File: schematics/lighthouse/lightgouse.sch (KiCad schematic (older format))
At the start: 4 parts

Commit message: lighthouse scheme
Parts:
- added D1, D2: LED, LEDs:LED-5MM, symbol LED
- added P1: 3V3, Pin_Headers:Pin_Header_Straight_1x01, symbol CONN_01X01
- added P2: GND, Pin_Headers:Pin_Header_Straight_1x01, symbol CONN_01X01
- added R1, R2: 1k, Resistors_ThroughHole:Resistor_Horizontal_RM7mm, symbol R
- added R5: 10k, w_pth_resistors:RC05, symbol R
- R3: renamed from 10k; value R -> 10K; footprint (none) -> w_pth_resistors:RC05
- R4: renamed from 10k; value R -> 10k; footprint (none) -> w_pth_resistors:RC05
- U1: renamed from U?; footprint (none) -> bugs:ESP201
- U2: renamed from U?; footprint (none) -> bugs:RC522
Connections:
- net labels removed: +3V3, GND
- wire segments 31 -> 41
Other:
- moved on the sheet: R3, R4, U2
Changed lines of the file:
@@
 EESchema Schematic File Version 2
+LIBS:lightgouse-rescue
 LIBS:power
 LIBS:device
@@
 $EndDescr
 $Comp
-L rc522 U?
+L rc522 U2
 U 1 1 5718CF80
-P 5250 2900
-F 0 "U?" H 5550 2950 60  0000 C CNN
-F 1 "rc522" H 5550 3100 60  0000 C CNN
-F 2 "" H 5150 3100 60  0000 C CNN
-F 3 "" H 5150 3100 60  0000 C CNN
-	1    5250 2900
+P 5800 2900
+F 0 "U2" H 6100 2950 60  0000 C CNN
+F 1 "rc522" H 6100 3100 60  0000 C CNN
+F 2 "bugs:RC522" H 5700 3100 60  0001 C CNN
+F 3 "" H 5700 3100 60  0000 C CNN
+	1    5800 2900
 	1    0    0    -1
 $EndComp
 $Comp
-L ESP-201 U?
+L R R4
+U 1 1 5718DD6D
+P 4000 3150
+F 0 "R4" V 3900 3150 50  0000 C CNN
+F 1 "10k" V 4000 3150 50  0000 C CNN
+F 2 "w_pth_resistors:RC05" V 3930 3150 50  0001 C CNN
+F 3 "" H 4000 3150 50  0000 C CNN
+	1    4000 3150
+	0    1    1    0
+$EndComp
+$Comp
+L R R3
+U 1 1 5718DDEA
+P 4000 2650
+F 0 "R3" V 4080 2650 50  0000 C CNN
+F 1 "10K" V 4000 2650 50  0000 C CNN
+F 2 "w_pth_resistors:RC05" V 3930 2650 50  0001 C CNN
+F 3 "" H 4000 2650 50  0000 C CNN
+	1    4000 2650
+	0    1    1    0
+$EndComp
+$Comp
+L R R5
+U 1 1 571A5ED5
+P 4000 3250
+F 0 "R5" V 4080 3250 50  0000 C CNN
+F 1 "10k" V 4000 3250 50  0000 C CNN
+F 2 "w_pth_resistors:RC05" V 3930 3250 50  0001 C CNN
+F 3 "" H 4000 3250 50  0000 C CNN
+	1    4000 3250
+	0    1    1    0
+$EndComp
+$Comp
+L CONN_01X01 P1
+U 1 1 571A6BF5
+P 3050 1350
+F 0 "P1" H 3050 1450 50  0000 C CNN
+F 1 "3V3" V 3150 1350 50  0000 C CNN
+F 2 "Pin_Headers:Pin_Header_Straight_1x01" H 3050 1350 50  0001 C CNN
+F 3 "" H 3050 1350 50  0000 C CNN
+	1    3050 1350
+	0    -1   -1   0
+$EndComp
+$Comp
+L CONN_01X01 P2
+U 1 1 571A6C6D
+P 3350 1350
+F 0 "P2" H 3350 1450 50  0000 C CNN
+F 1 "GND" V 3450 1350 50  0000 C CNN
+F 2 "Pin_Headers:Pin_Header_Straight_1x01" H 3350 1350 50  0001 C CNN
+F 3 "" H 3350 1350 50  0000 C CNN
+	1    3350 1350
+	0    -1   -1   0
+$EndComp
+$Comp
+L LED D2
+U 1 1 571A6EF4
+P 2050 3200
+F 0 "D2" H 2050 3300 50  0000 C CNN
+F 1 "LED" H 2050 3100 50  0000 C CNN
+F 2 "LEDs:LED-5MM" H 2050 3200 50  0001 C CNN
+F 3 "" H 2050 3200 50  0000 C CNN
+	1    2050 3200
+	0    1    1    0
+$EndComp
+$Comp
+L LED D1
+U 1 1 571A6FA0
+P 2150 2450
+F 0 "D1" H 2150 2550 50  0000 C CNN
+F 1 "LED" H 2150 2350 50  0000 C CNN
+F 2 "LEDs:LED-5MM" H 2150 2450 50  0001 C CNN
+F 3 "" H 2150 2450 50  0000 C CNN
+	1    2150 2450
+	0    1    1    0
+$EndComp
+$Comp
+L R R2
+U 1 1 571A710A
+P 2400 2650
+F 0 "R2" V 2480 2650 50  0000 C CNN
+F 1 "1k" V 2400 2650 50  0000 C CNN
+F 2 "Resistors_ThroughHole:Resistor_Horizontal_RM7mm" V 2330 2650 50  0001 C CNN
+F 3 "" H 2400 2650 50  0000 C CNN
+	1    2400 2650
+	0    1    1    0
+$EndComp
+$Comp
+L R R1
+U 1 1 571A724A
+P 2350 3450
+F 0 "R1" V 2430 3450 50  0000 C CNN
+F 1 "1k" V 2350 3450 50  0000 C CNN
+F 2 "Resistors_ThroughHole:Resistor_Horizontal_RM7mm" V 2280 3450 50  0001 C CNN
+F 3 "" H 2350 3450 50  0000 C CNN
+	1    2350 3450
+	0    1    1    0
+$EndComp
+$Comp
+L ESP-201 U1
 U 1 1 5718D2DA
 P 3200 3150
-F 0 "U?" H 3300 3300 60  0000 C CNN
+F 0 "U1" H 3300 3300 60  0000 C CNN
 F 1 "ESP-201" H 3200 3450 60  0000 C CNN
-F 2 "" H 3450 3350 60  0000 C CNN
+F 2 "bugs:ESP201" H 3450 3350 60  0001 C CNN
 F 3 "" H 3450 3350 60  0000 C CNN
 	1    3200 3150
@@
 	4700 2550 4700 1950
 Wire Wire Line
-	4700 1950 2200 1950
-Wire Wire Line
-	2200 1950 2200 2750
-Wire Wire Line
-	2200 2750 2600 2750
-Wire Wire Line
-	3800 2750 4700 2750
+	4700 1950 1950 1950
+Wire Wire Line
+	1950 1950 1950 2750
+Wire Wire Line
+	1950 2750 2600 2750
+Wire Wire Line
+	3800 2750 5250 2750
 Wire Wire Line
 	3800 2950 4400 2950
 Wire Wire Line
-	3800 2850 4700 2850
-Wire Wire Line
-	4700 3900 4700 3250
-Wire Wire Line
-	2600 3900 4700 3900
+	3800 2850 5250 2850
+Wire Wire Line
+	4950 3900 4950 3250
+Wire Wire Line
+	2600 3900 4950 3900
 Wire Wire Line
 	2600 3900 2600 3650
 Wire Wire Line
+	4350 3050 4350 3550
+Wire Wire Line
+	4350 3550 3800 3550
+Wire Wire Line
+	3050 1550 3050 2300
+Wire Wire Line
+	3350 1550 3350 2300
+Wire Wire Line
+	4550 3150 5250 3150
+Wire Wire Line
+	4250 2150 4250 3250
+Wire Wire Line
+	5250 2550 4700 2550
+Wire Wire Line
+	4250 3250 4150 3250
+Wire Wire Line
+	4250 3150 4150 3150
+Wire Wire Line
+	3850 3150 3800 3150
+Wire Wire Line
+	3800 3250 3850 3250
+Connection ~ 4250 3150
+Connection ~ 3050 2150
+Wire Wire Line
+	2550 2650 2600 2650
+Wire Wire Line
+	2050 2200 4150 2200
+Wire Wire Line
+	4150 2200 4150 2650
+Connection ~ 3350 2200
+Wire Wire Line
+	3850 2650 3800 2650
+Wire Wire Line
+	3050 2150 4250 2150
+Wire Wire Line
+	2050 3000 2050 2200
+Connection ~ 2150 2200
+Wire Wire Line
+	4550 3450 3800 3450
+Wire Wire Line
+	4550 3150 4550 3450
+Wire Wire Line
+	2500 3450 2600 3450
+Wire Wire Line
+	2550 3550 2600 3550
+Wire Wire Line
+	2050 3450 2200 3450
+Wire Wire Line
+	2050 3400 2050 3450
+Wire Wire Line
+	2150 2250 2150 2200
+Wire Wire Line
+	2250 2650 2150 2650
+Wire Wire Line
 	4400 2950 4400 2650
 Wire Wire Line
-	4400 2650 4700 2650
-Wire Wire Line
-	4700 3050 3950 3050
-Wire Wire Line
-	3950 3050 3950 3550
-Wire Wire Line
-	3950 3550 3800 3550
-$Comp
-L +3V3 #PWR?
-U 1 1 5718DC65
-P 3050 1650
-F 0 "#PWR?" H 3050 1500 50  0001 C CNN
-F 1 "+3V3" H 3050 1790 50  0000 C CNN
-F 2 "" H 3050 1650 50  0000 C CNN
-F 3 "" H 3050 1650 50  0000 C CNN
-	1    3050 1650
-	1    0    0    -1
-$EndComp
-Wire Wire Line
-	3050 1650 3050 2300
-$Comp
-L GND #PWR?
-U 1 1 5718DCCC
-P 3350 1650
-F 0 "#PWR?" H 3350 1400 50  0001 C CNN
-F 1 "GND" H 3350 1500 50  0000 C CNN
-F 2 "" H 3350 1650 50  0000 C CNN
-F 3 "" H 3350 1650 50  0000 C CNN
-	1    3350 1650
-	-1   0    0    1
-$EndComp
-Wire Wire Line
-	3350 1650 3350 2300
-Wire Wire Line
-	4750 3150 4200 3150
-Wire Wire Line
-	4200 3150 4200 3850
-Wire Wire Line
-	4200 3850 2500 3850
-Wire Wire Line
-	2500 3850 2500 3450
-Wire Wire Line
-	2500 3450 2600 3450
-$Comp
-L R 10k
-U 1 1 5718DD6D
-P 2850 1800
-F 0 "10k" V 2930 1800 50  0000 C CNN
-F 1 "R" V 2850 1800 50  0000 C CNN
-F 2 "" V 2780 1800 50  0000 C CNN
-F 3 "" H 2850 1800 50  0000 C CNN
-	1    2850 1800
-	0    1    1    0
-$EndComp
-Wire Wire Line
-	3000 1800 3050 1800
-Connection ~ 3050 1800
-Wire Wire Line
-	3800 3150 3900 3150
-Wire Wire Line
-	3900 3150 3900 1350
-Wire Wire Line
-	3900 1350 2650 1350
-Wire Wire Line
-	2650 1350 2650 1800
-Wire Wire Line
-	2650 1800 2700 1800
-$Comp
-L R 10k
-U 1 1 5718DDEA
-P 3550 1800
-F 0 "10k" V 3630 1800 50  0000 C CNN
-F 1 "R" V 3550 1800 50  0000 C CNN
-F 2 "" V 3480 1800 50  0000 C CNN
-F 3 "" H 3550 1800 50  0000 C CNN
-	1    3550 1800
-	0    1    1    0
-$EndComp
-Wire Wire Line
-	3400 1800 3350 1800
-Connection ~ 3350 1800
-Wire Wire Line
-	3700 1800 3800 1800
-Wire Wire Line
-	3800 1800 3800 2650
+	4400 2650 5250 2650
+Wire Wire Line
+	4350 3050 5250 3050
+Wire Wire Line
+	5250 3250 5150 3250
+Wire Wire Line
+	5150 3250 5150 1750
+Wire Wire Line
+	5150 1750 3050 1750
+Connection ~ 3050 1750
 $EndSCHEMATC

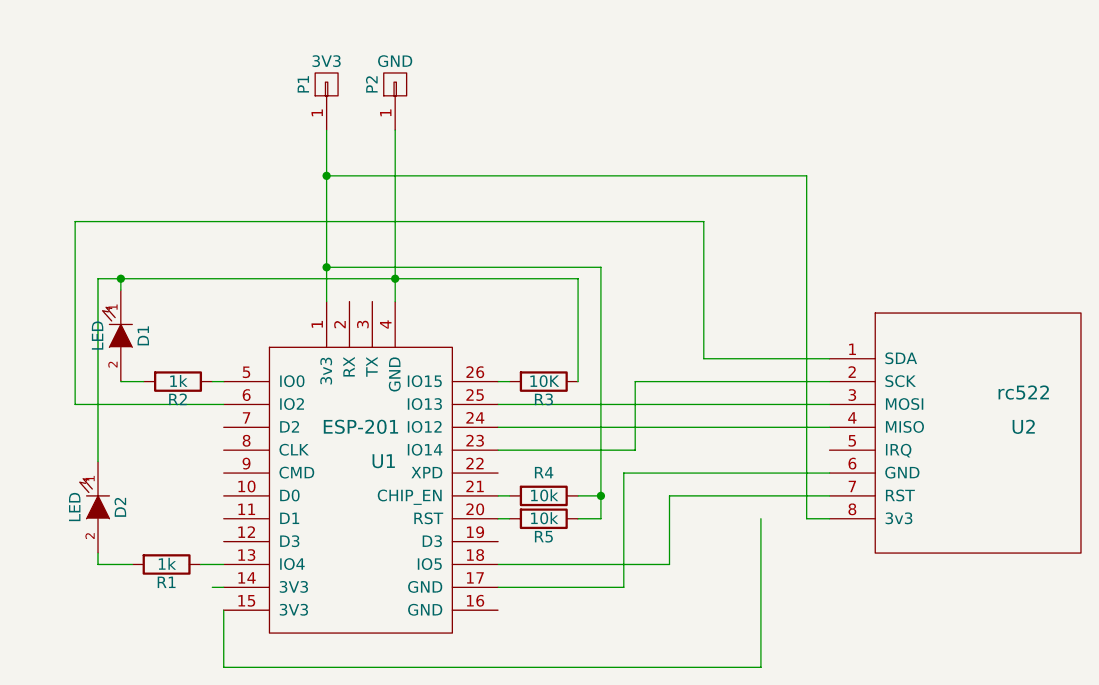
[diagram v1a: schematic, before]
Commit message: lighthouse schematic update
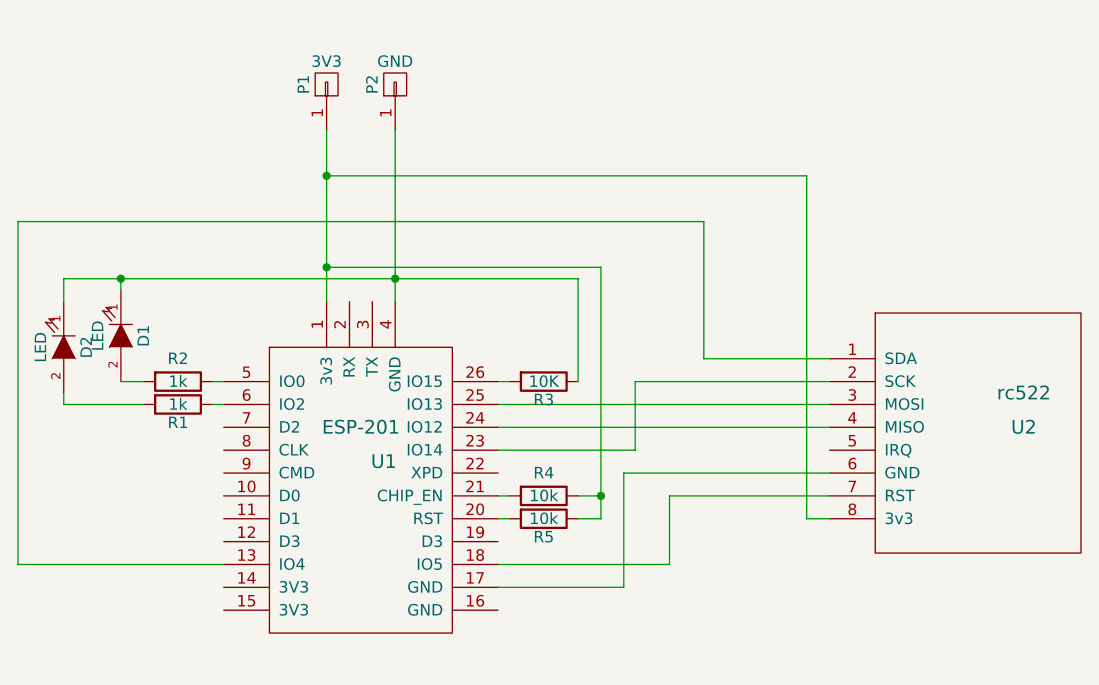
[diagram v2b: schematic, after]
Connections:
- wire segments 41 -> 37
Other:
- moved on the sheet: D2, R1
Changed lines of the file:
@@
 L LED D2
 U 1 1 571A6EF4
-P 2050 3200
-F 0 "D2" H 2050 3300 50  0000 C CNN
-F 1 "LED" H 2050 3100 50  0000 C CNN
-F 2 "LEDs:LED-5MM" H 2050 3200 50  0001 C CNN
-F 3 "" H 2050 3200 50  0000 C CNN
-	1    2050 3200
+P 1900 2500
+F 0 "D2" H 1900 2600 50  0000 C CNN
+F 1 "LED" H 1900 2400 50  0000 C CNN
+F 2 "LEDs:LED-5MM" H 1900 2500 50  0001 C CNN
+F 3 "" H 1900 2500 50  0000 C CNN
+	1    1900 2500
 	0    1    1    0
 $EndComp
@@
 U 1 1 571A710A
 P 2400 2650
-F 0 "R2" V 2480 2650 50  0000 C CNN
+F 0 "R2" V 2300 2650 50  0000 C CNN
 F 1 "1k" V 2400 2650 50  0000 C CNN
 F 2 "Resistors_ThroughHole:Resistor_Horizontal_RM7mm" V 2330 2650 50  0001 C CNN
@@
 L R R1
 U 1 1 571A724A
-P 2350 3450
-F 0 "R1" V 2430 3450 50  0000 C CNN
-F 1 "1k" V 2350 3450 50  0000 C CNN
-F 2 "Resistors_ThroughHole:Resistor_Horizontal_RM7mm" V 2280 3450 50  0001 C CNN
-F 3 "" H 2350 3450 50  0000 C CNN
-	1    2350 3450
+P 2400 2750
+F 0 "R1" V 2480 2750 50  0000 C CNN
+F 1 "1k" V 2400 2750 50  0000 C CNN
+F 2 "Resistors_ThroughHole:Resistor_Horizontal_RM7mm" V 2330 2750 50  0001 C CNN
+F 3 "" H 2400 2750 50  0000 C CNN
+	1    2400 2750
 	0    1    1    0
 $EndComp
@@
 $EndComp
 Wire Wire Line
-	4700 2550 4700 1950
+	4700 1950 4700 2550
 Wire Wire Line
-	4700 1950 1950 1950
-Wire Wire Line
-	1950 1950 1950 2750
-Wire Wire Line
-	1950 2750 2600 2750
+	1700 1950 4700 1950
 Wire Wire Line
 	3800 2750 5250 2750
@@
 Wire Wire Line
 	3800 2850 5250 2850
-Wire Wire Line
-	4950 3900 4950 3250
-Wire Wire Line
-	2600 3900 4950 3900
-Wire Wire Line
-	2600 3900 2600 3650
 Wire Wire Line
 	4350 3050 4350 3550
@@
 	4250 2150 4250 3250
 Wire Wire Line
-	5250 2550 4700 2550
+	4700 2550 5250 2550
 Wire Wire Line
 	4250 3250 4150 3250
@@
 	2550 2650 2600 2650
 Wire Wire Line
-	2050 2200 4150 2200
+	1900 2200 4150 2200
 Wire Wire Line
 	4150 2200 4150 2650
@@
 Wire Wire Line
 	3050 2150 4250 2150
-Wire Wire Line
-	2050 3000 2050 2200
 Connection ~ 2150 2200
 Wire Wire Line
@@
 Wire Wire Line
 	4550 3150 4550 3450
-Wire Wire Line
-	2500 3450 2600 3450
-Wire Wire Line
-	2550 3550 2600 3550
-Wire Wire Line
-	2050 3450 2200 3450
-Wire Wire Line
-	2050 3400 2050 3450
 Wire Wire Line
 	2150 2250 2150 2200
@@
 	5150 1750 3050 1750
 Connection ~ 3050 1750
+Wire Wire Line
+	2550 2750 2600 2750
+Wire Wire Line
+	1900 2700 1900 2750
+Wire Wire Line
+	1900 2750 2250 2750
+Wire Wire Line
+	1900 2300 1900 2200
+Wire Wire Line
+	1700 1950 1700 3450
+Wire Wire Line
+	1700 3450 2600 3450
 $EndSCHEMATC
